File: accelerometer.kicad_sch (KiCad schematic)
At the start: 9 parts, among them U801 LIS3DHTR

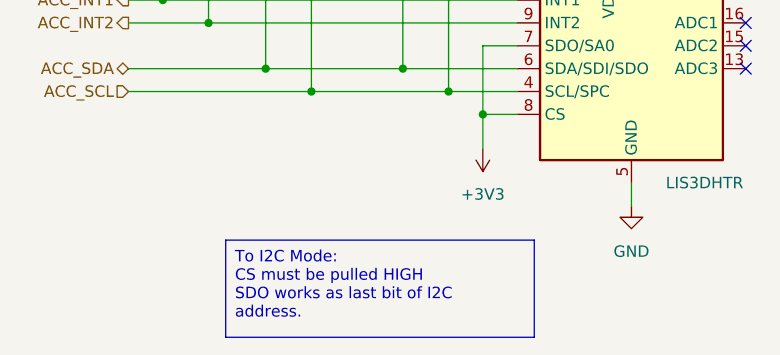
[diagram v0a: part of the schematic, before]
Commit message: small fixes
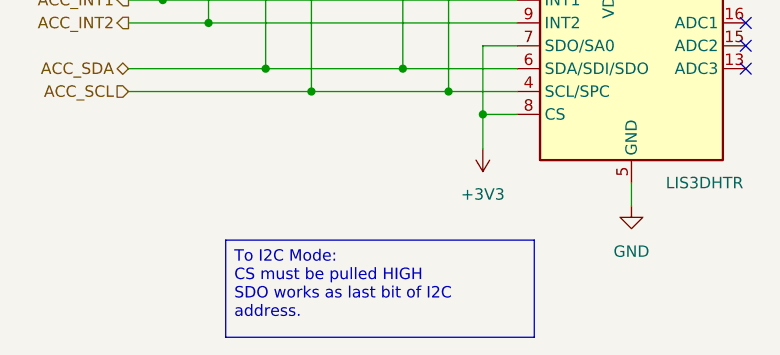
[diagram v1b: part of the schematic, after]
